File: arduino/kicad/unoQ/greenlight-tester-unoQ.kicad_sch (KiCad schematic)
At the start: 37 parts, among them J1 AudioJack2, J1 Conn_01x08, J2 AudioJack2, J2 Conn_01x08, J3 Conn_01x10, J3 XLR3, J4 Conn_01x08, J4 XLR3, J5 Conn_01x08, J6 Conn_01x08, K1 Relay_DPDT, K2 Relay_DPDT, K3 Relay_DPDT, K4 Relay_DPDT, K5 Relay_DPDT, K6 Relay_DPDT, Q1 PN2222A, SW1 SW_Push

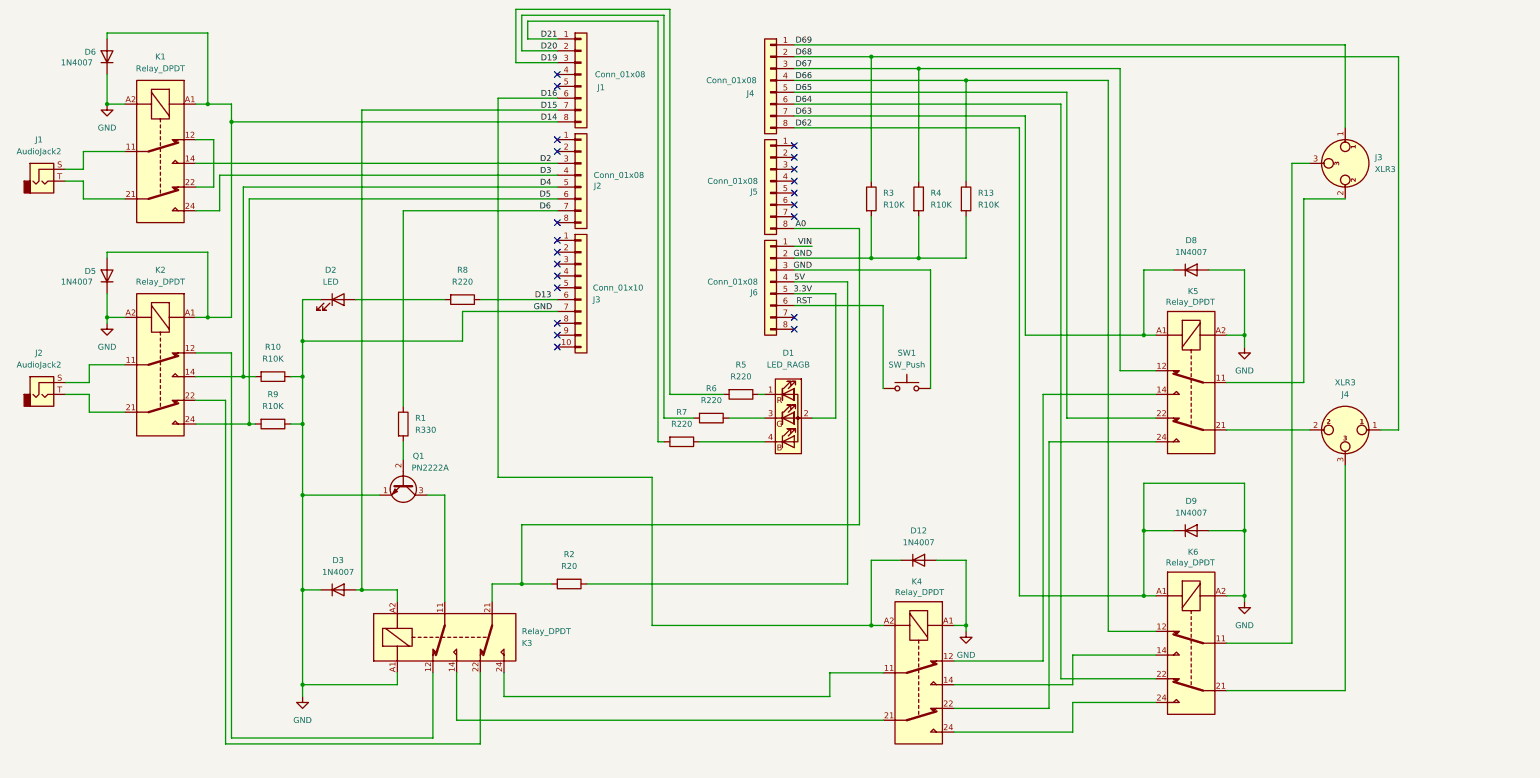
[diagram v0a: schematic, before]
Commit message: kicad updates, puzzle light map, more util updates
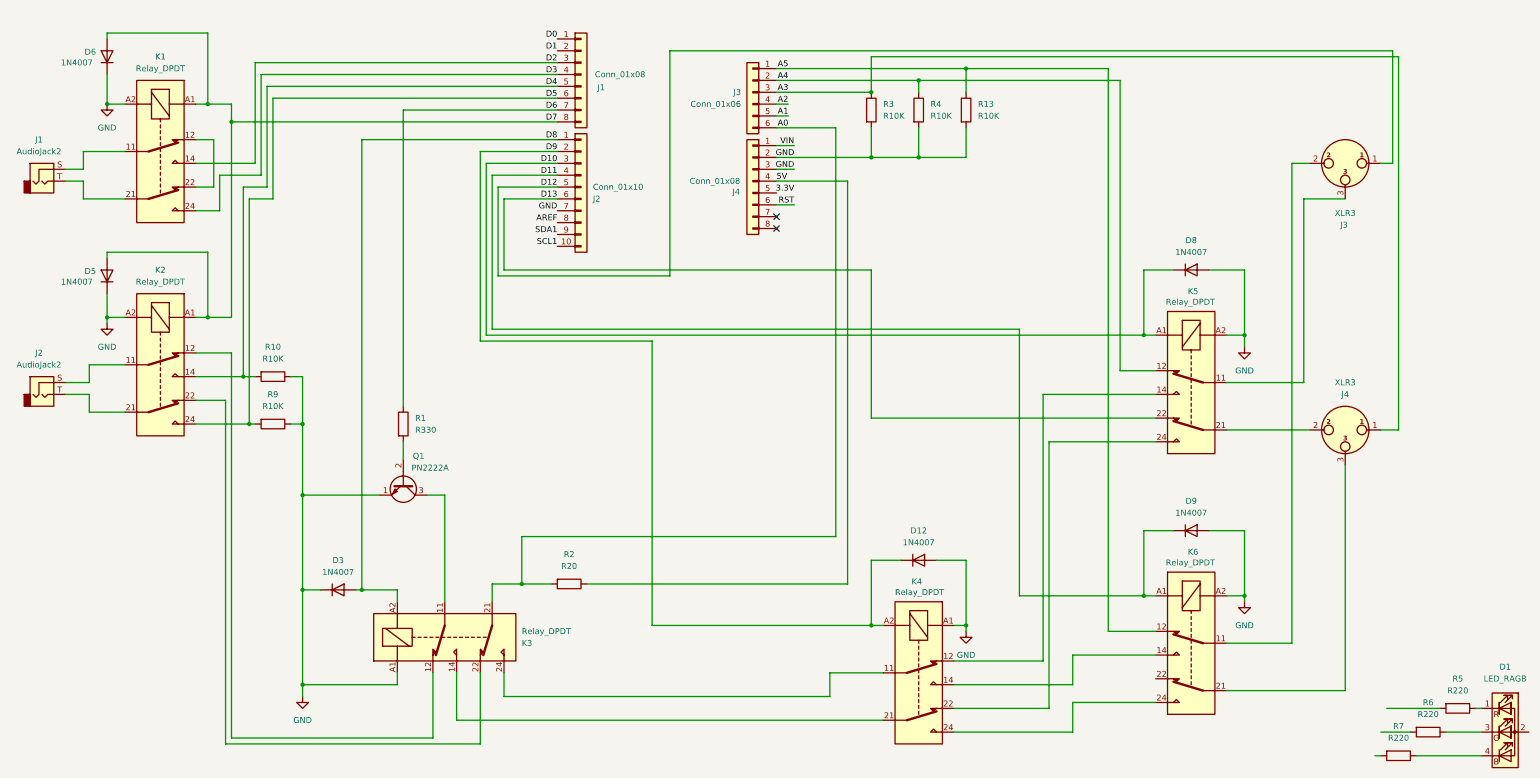
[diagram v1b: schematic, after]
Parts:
- removed D2: LED, symbol Device:LED
- removed J2, J4, J5: Conn_01x08, symbol Connector_Generic:Conn_01x08
- removed R8: R220, Resistor_THT:R_Axial_DIN0204_L3.6mm_D1.6mm_P1.90mm_Vertical, symbol Device:R
- removed SW1: SW_Push, Connector_PinHeader_2.54mm:PinHeader_1x02_P2.54mm_Vertical, symbol Switch:SW_Push
- added J3: Conn_01x06, symbol Connector_Generic:Conn_01x06
- renumbered J3 to J2, J6 to J4
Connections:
- net D63 is gone; now on net D10: D8.1 (K), K5.A1
- net D65 is gone; now on net D13: K5.22
- net D69 is gone; now on net D12: J3.1
- net 3.3V: no longer D1.2 (A), J4.5 (+3V3)
- net A0: now also J3.6 (A0)
- net D2: now also J1.3 (D2)
- net D3: now also J1.4 (D3)
- net D4: now also J1.5 (D4)
- net D5: now also J1.6 (D5)
- net D6: now also J1.7 (D6)
- net GND: no longer D9.1 (K), K6.A1
- net at J3.2: now also K6.11; no longer K5.11
- net at J3.3: now also K5.11; no longer K6.11
- net D8: now reaches J2.1 (D8)
- net D8: now also D3.2 (A), K3.A2
- net SCL1: now reaches J2.10 (SCL1)
- net D9: now reaches J2.2 (D9)
- net D9: now also D12.1 (K), K4.A2
- net D10: now reaches J2.3 (D10)
- net D11: now reaches J2.4 (D11)
- net D11: now also D9.1 (K), K6.A1
- net D12: now reaches J2.5 (D12)
- net AREF: now reaches J2.8 (AREF)
- net SDA1: now reaches J2.9 (SDA1)
- net D14 renamed D7
- removed net D15: D3.2 (A), J1.7 (D15), K3.A2
- removed net D16: D12.1 (K), J1.6 (D16), K4.A2
- net D19: no longer names the net of R5.2
- net D19: no longer J1.3 (D19)
- net D20: no longer names the net of R6.2
- net D20: no longer J1.2 (D20)
- net D21: no longer names the net of R7.2
- net D21: no longer J1.1 (D21)
- net D64: no longer names the net of K6.22
- net D66 renamed A5
- net A5: now also J3.1 (A5)
- net D67 renamed A4
- net A4: now also J3.2 (A4)
- net D68 renamed A3
- net A3: now also J3.3 (A3)
- new net A1: J3.5 (A1)
- new net A2: J3.4 (A2)
- new net D0: J1.1 (D0)
- new net D1: J1.2 (D1)
- no-connect marks 22 -> 2
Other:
- moved on the sheet: D1, J2, J4, R13, R3, R4, R5, R6, R7
